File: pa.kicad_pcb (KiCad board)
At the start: 2 copper layers, 100.3 x 71.1 mm, 91 parts, among them J1 Conn_Coaxial, J10 TX5V, J11 12V-PA, J12 12V, J2 20m, J3 40m, J4 80m, J5 Key5V, J6 RX-HF, J7 TX-HF, J8 12V, J9 10m, K1 FINDER-30.22, K2 FINDER-30.22, K3 FINDER-30.22, K4 FINDER-30.22, Q1 2N3904, Q10 2N3904, Q11 BS170, Q2 2N3904, Q3 2N3904, Q4 BS170, Q5 BD140, Q6 BS170, Q7 BS170, Q8 BS170, Q9 BS170, T1 8+8@FT37-43, U1 74HCT00, U2 L78L05_TO92

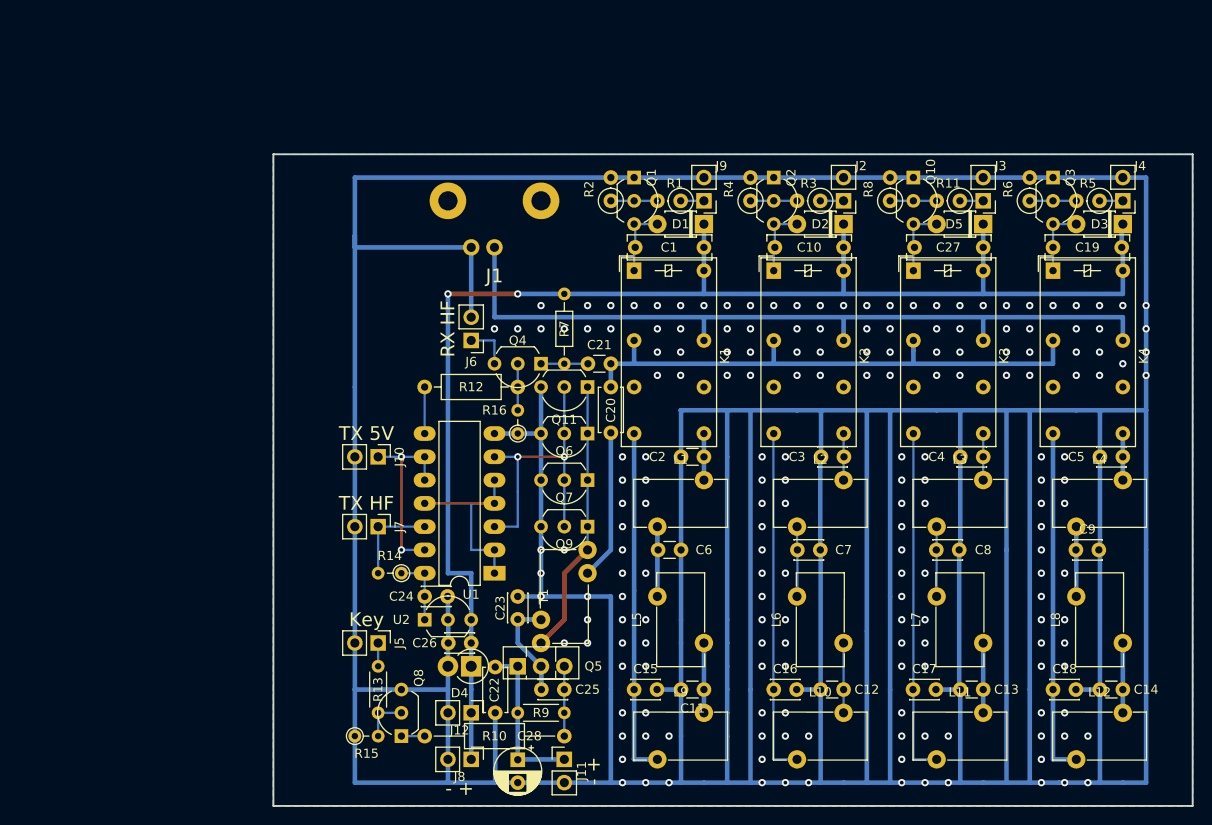
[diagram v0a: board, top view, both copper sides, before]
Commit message: Added revision 2 hardware.
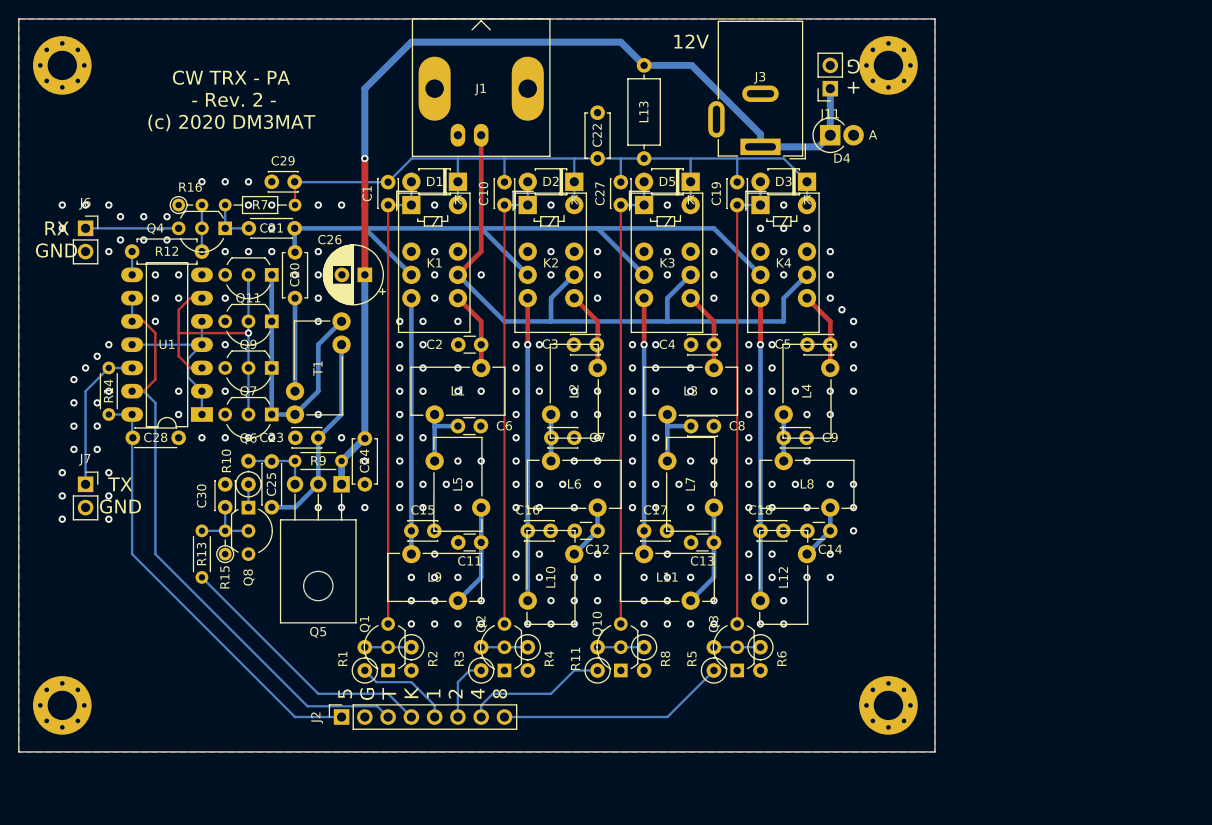
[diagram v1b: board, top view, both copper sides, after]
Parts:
- removed J10: TX5V, Connector_PinHeader_2.54mm:PinHeader_1x02_P2.54mm_Vertical
- removed J12, J8: 12V, Connector_PinHeader_2.54mm:PinHeader_1x02_P2.54mm_Vertical
- removed J4: 80m, Connector_PinHeader_2.54mm:PinHeader_1x02_P2.54mm_Vertical
- removed J5: Key5V, Connector_PinHeader_2.54mm:PinHeader_1x02_P2.54mm_Vertical
- removed J9: 10m, Connector_PinHeader_2.54mm:PinHeader_1x02_P2.54mm_Vertical
- removed U2: L78L05_TO92, Package_TO_SOT_THT:TO-92_Inline_Wide
- added C29: 100n, Capacitor_THT:C_Disc_D3.0mm_W2.0mm_P2.50mm, F.Cu at (97.6, 67.8)
- added C30: 100n, Capacitor_THT:C_Disc_D3.0mm_W2.0mm_P2.50mm, F.Cu at (92.5, 100.8)
- added H1: GND, MountingHole:MountingHole_3.2mm_M3_Pad_Via, F.Cu at (164.9, 124.9)
- added H2: GND, MountingHole:MountingHole_3.2mm_M3_Pad_Via, F.Cu at (164.9, 55.1)
- added H3: GND, MountingHole:MountingHole_3.2mm_M3_Pad_Via, F.Cu at (74.8, 55.1)
- added H4: GND, MountingHole:MountingHole_3.2mm_M3_Pad_Via, F.Cu at (74.8, 124.9)
- added L13: 100u, Inductor_THT:L_Axial_L7.0mm_D3.3mm_P10.16mm_Horizontal_Fastron_MICC, F.Cu at (138.2, 65.2)
- C1, C10, C19, C27: footprint Capacitor_THT:C_Rect_L9.0mm_W2.5mm_P7.50mm_MKT -> Capacitor_THT:C_Disc_D3.0mm_W2.0mm_P2.50mm
- C21: footprint Capacitor_THT:C_Disc_D3.0mm_W1.6mm_P2.50mm -> Capacitor_THT:C_Disc_D4.3mm_W1.9mm_P5.00mm
- C24: footprint Capacitor_THT:C_Disc_D3.0mm_W2.0mm_P2.50mm -> Capacitor_THT:C_Disc_D4.7mm_W2.5mm_P5.00mm
- C25: footprint Capacitor_THT:C_Disc_D3.0mm_W2.0mm_P2.50mm -> Capacitor_THT:C_Disc_D4.3mm_W1.9mm_P5.00mm
- C26: value 100n -> 220u; footprint Capacitor_THT:C_Disc_D3.0mm_W2.0mm_P2.50mm -> Capacitor_THT:CP_Radial_D6.3mm_P2.50mm
- C28: value 100u -> 100n; footprint Capacitor_THT:CP_Radial_D5.0mm_P2.50mm -> Capacitor_THT:C_Disc_D4.3mm_W1.9mm_P5.00mm
- J1: footprint Connector_Coaxial:BNC_horizontal -> Connector_Coaxial:BNC_Amphenol_B6252HB-NPP3G-50_Horizontal
- J11: value 12V-PA -> RXSupply; footprint Connector_PinHeader_2.54mm:PinHeader_1x02_P2.54mm_Vertical -> Connector_PinSocket_2.54mm:PinSocket_1x02_P2.54mm_Vertical
- J2: value 20m -> FromRX; footprint Connector_PinHeader_2.54mm:PinHeader_1x02_P2.54mm_Vertical -> Connector_PinSocket_2.54mm:PinSocket_1x08_P2.54mm_Vertical
- J3: value 40m -> Barrel_Jack_Switch; footprint Connector_PinHeader_2.54mm:PinHeader_1x02_P2.54mm_Vertical -> Connector_BarrelJack:BarrelJack_Wuerth_6941xx301002
- J6, J7: footprint Connector_PinHeader_2.54mm:PinHeader_1x02_P2.54mm_Vertical -> Connector_PinSocket_2.54mm:PinSocket_1x02_P2.54mm_Vertical
- K1, K2, K3, K4: value FINDER-30.22 -> G6S-2; footprint Relay_THT:Relay_DPDT_Finder_30.22 -> Relay_THT:Relay_DPDT_Omron_G6S-2
- L1, L3, L5, L7: footprint Inductor_THT:L_Toroid_Vertical_L10.0mm_W5.0mm_P5.08mm_Diagonal -> DM3MAT:L_Toroid_Vertical_L10.0mm_W5.0mm_P5.08mm_Diagonal_Rev
- L10, L11, L12, L2, L4, L6, L8, L9: footprint Inductor_THT:L_Toroid_Vertical_L10.0mm_W5.0mm_P5.08mm_Diagonal -> DM3MAT:L_Toroid_Vertical_L10.0mm_W5.0mm_P5.08mm_Diagonal
- Q5: footprint Package_TO_SOT_THT:TO-126-3_Vertical -> Package_TO_SOT_THT:TO-126-3_Horizontal_TabDown
- R10: footprint Resistor_THT:R_Axial_DIN0207_L6.3mm_D2.5mm_P15.24mm_Horizontal -> Resistor_THT:R_Axial_DIN0207_L6.3mm_D2.5mm_P2.54mm_Vertical
- R12: footprint Resistor_THT:R_Axial_DIN0207_L6.3mm_D2.5mm_P10.16mm_Horizontal -> Resistor_THT:R_Axial_DIN0207_L6.3mm_D2.5mm_P7.62mm_Horizontal
- R14: footprint Resistor_THT:R_Axial_DIN0204_L3.6mm_D1.6mm_P2.54mm_Vertical -> Resistor_THT:R_Axial_DIN0204_L3.6mm_D1.6mm_P5.08mm_Horizontal
- moved J11 78.7 mm to (158.6, 57.6), turned to 180 degrees
- moved J2 78.6 mm to (105.2, 126.2), turned to 90 degrees
- moved D4 70.0 mm to (158.6, 62.7), turned to 0 degrees
- moved C22 66.4 mm to (133.2, 60.2), turned to 270 degrees
- moved R5 66.3 mm to (145.9, 121.1), turned to 90 degrees
- moved R11 64.7 mm to (133.2, 121.1), turned to 90 degrees
- moved Q3 63.9 mm to (148.4, 121.1), turned to 90 degrees
- moved R3 63.2 mm to (120.5, 121.1), turned to 90 degrees
- moved Q10 62.6 mm to (135.7, 121.1), turned to 90 degrees
- moved R1 61.8 mm to (107.8, 121.1), turned to 90 degrees
- moved Q2 61.3 mm to (123.0, 121.1), turned to 90 degrees
- moved Q1 60.1 mm to (110.3, 121.1), turned to 90 degrees
- moved R6 56.9 mm to (150.9, 118.6), turned to 270 degrees
- moved R8 55.6 mm to (138.2, 118.6), turned to 270 degrees
- moved R4 54.4 mm to (125.5, 118.6), turned to 270 degrees
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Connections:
- C22 pad 2: VCC -> +12V
- C24 pad 2: +5V -> VCC
- C26 pad 1: GND -> VCC
- C26 pad 2: +12V -> GND
- C28 pad 1: VCC -> GND
- C28 pad 2: GND -> +5V
- D4 pad 1: +12V -> VCC
- J2 pad 1: 20m -> +5V
- J3 pad 1: 40m -> VCC
- K1 pad 12: Net-(K1-Pad12) -> +12V
- K2 pad 12: Net-(K2-Pad12) -> +12V
- K3 pad 12: Net-(K3-Pad12) -> +12V
- K4 pad 12: Net-(K4-Pad12) -> +12V
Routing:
- net GND: track 892.3 -> 0.00 mm, vias 189 -> 236
- net VCC: track 17.8 -> 109.3 mm, vias 0 -> 1
- net +12V: track 157.6 -> 86.1 mm, vias 2 -> 0
- net TX5V: track 20.3 -> 66.1 mm, vias 2 -> 0
- net RL80M: track 7.62 -> 50.8 mm
- net RL20M: track 7.72 -> 50.8 mm
- net RL10M: track 7.72 -> 50.8 mm
- net RL40M: track 7.72 -> 50.8 mm
- net +5V: track 7.62 -> 48.0 mm
- net KEY5V: track 2.54 -> 29.2 mm
- net 80m: track 2.54 -> 25.0 mm
- net LPF: track 61.0 -> 77.1 mm
- net Net-(J1-Pad1): track 86.4 -> 72.4 mm
- net 40m: track 2.54 -> 15.5 mm
- net Net-(C23-Pad2): track 11.5 -> 22.4 mm
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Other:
- board size 100.3 x 71.1 mm -> 100 x 80 mm
- net class GND removed
- net class PWR added: clearance 0.2, trace_width 0.75, via_dia 0.8, via_drill 0.4
- net class RF added: clearance 0.2, trace_width 0.5, via_dia 0.8, via_drill 0.4
- board text added: "+ G"
- board text added: "12V"
- board text added: "5 G T K 1 2 4 8"
- board text added: "CW TRX - PA - Rev. 2 - (c) 2020 DM3MAT"
- board text added: "RX GND"
- board text added: "TX GND"
- board text removed: "- +"
- board text removed: "Key"
- board text removed: "RX HF"
- board text removed: "TX 5V"
- board text removed: "TX HF"
